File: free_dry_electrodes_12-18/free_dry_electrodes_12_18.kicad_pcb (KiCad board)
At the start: 2 copper layers, 14 x 14 mm, 30 parts

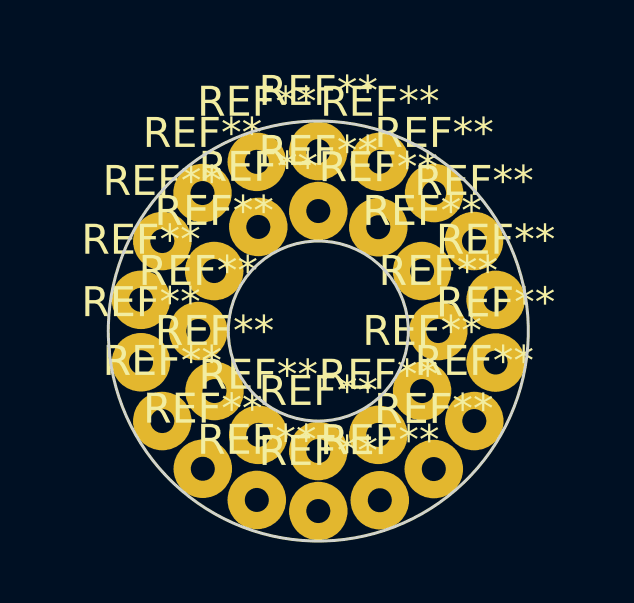
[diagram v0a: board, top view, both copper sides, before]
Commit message: Add files via upload
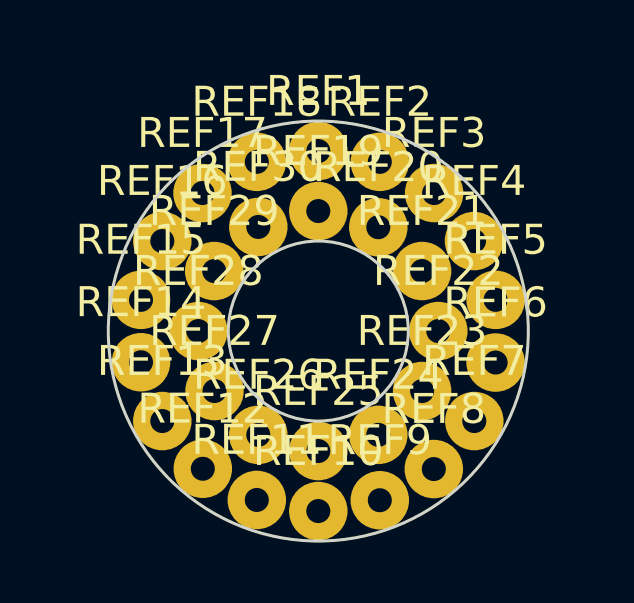
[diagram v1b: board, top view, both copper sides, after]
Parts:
- renumbered REF** to REF1, REF** to REF10, REF** to REF11, REF** to REF12, REF** to REF13, REF** to REF14, REF** to REF15, REF** to REF16, REF** to REF17, REF** to REF18, REF** to REF19, REF** to REF2, REF** to REF20, REF** to REF21, REF** to REF22, REF** to REF23, REF** to REF24, REF** to REF25, REF** to REF26, REF** to REF27, REF** to REF28, REF** to REF29, REF** to REF3, REF** to REF30, REF** to REF4, REF** to REF5, REF** to REF6, REF** to REF7, REF** to REF8, REF** to REF9
